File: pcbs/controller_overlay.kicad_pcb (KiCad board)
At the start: 2 copper layers, 19.7 x 60.1 mm, 2 parts

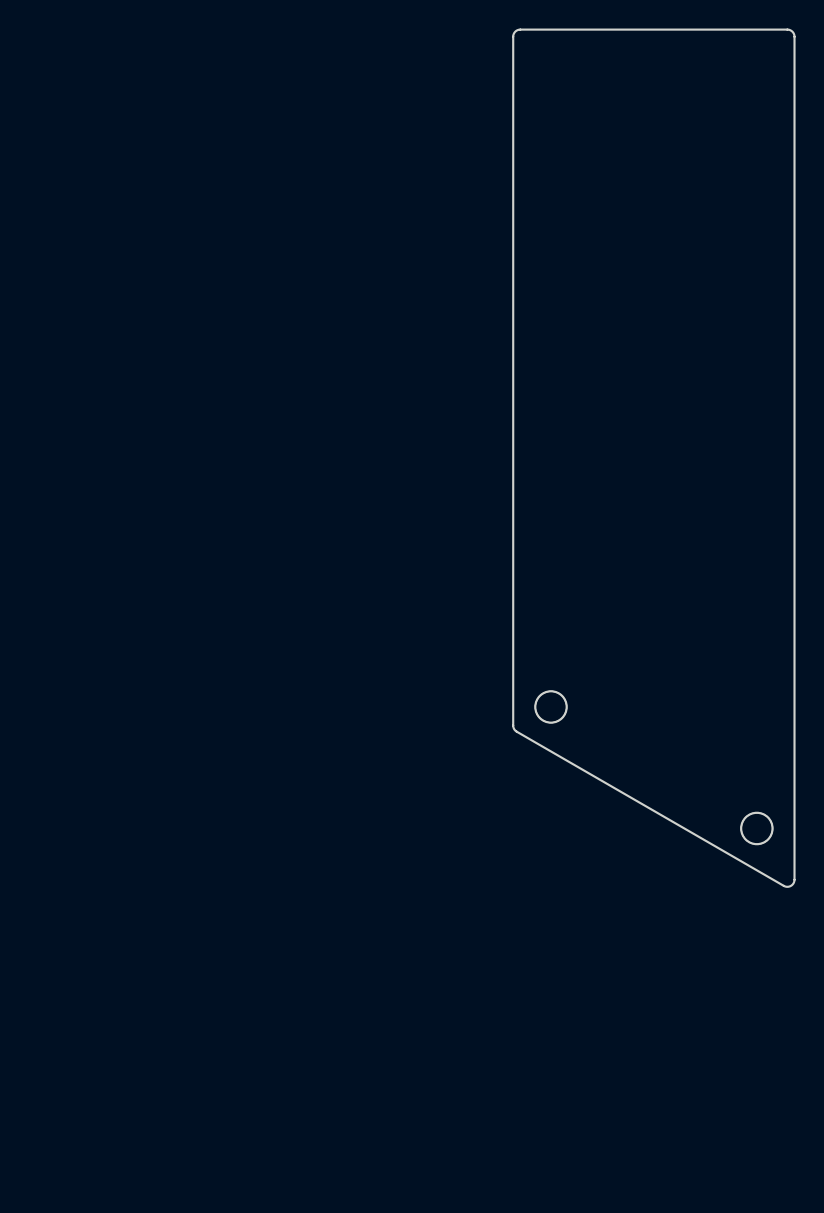
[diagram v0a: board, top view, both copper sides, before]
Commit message: First commit? Second?
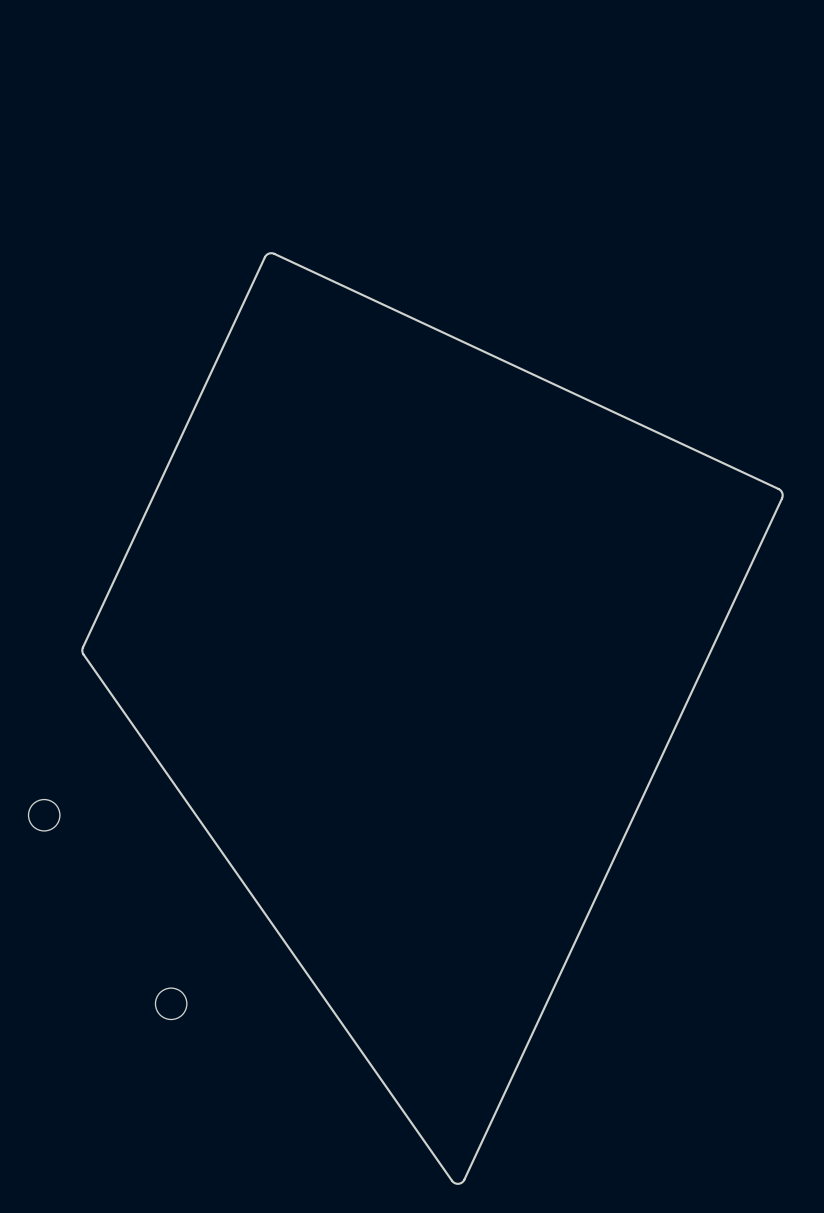
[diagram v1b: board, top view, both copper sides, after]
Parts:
- moved MH2 42.9 mm to (181.1, 121.3), turned to -25 degrees
- moved MH1 36.3 mm to (172.2, 108.1), turned to -25 degrees
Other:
- board size 19.7 x 60.1 mm -> 49.1 x 65.2 mm
